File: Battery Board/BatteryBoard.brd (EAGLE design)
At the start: 40.6 x 80.5 mm, 38 parts, among them IC1 TPS63060DSCT, J0 1725656, J1 1725669, J2 UJ2-MIBH2-4-SMT-TR, J3 MPTC-02-16-02-6.30-XX-X-V, J4 JSTPH2, J5 MPTC-02-04-02-6.30-XX-X-V-LC, Q1 MMBTA56LT1G, Q2 MMBTA56LT1G, U0 STM32L031K4U6, U1 MCP73831T-2ATI_OT, U3 STM809TWX6F

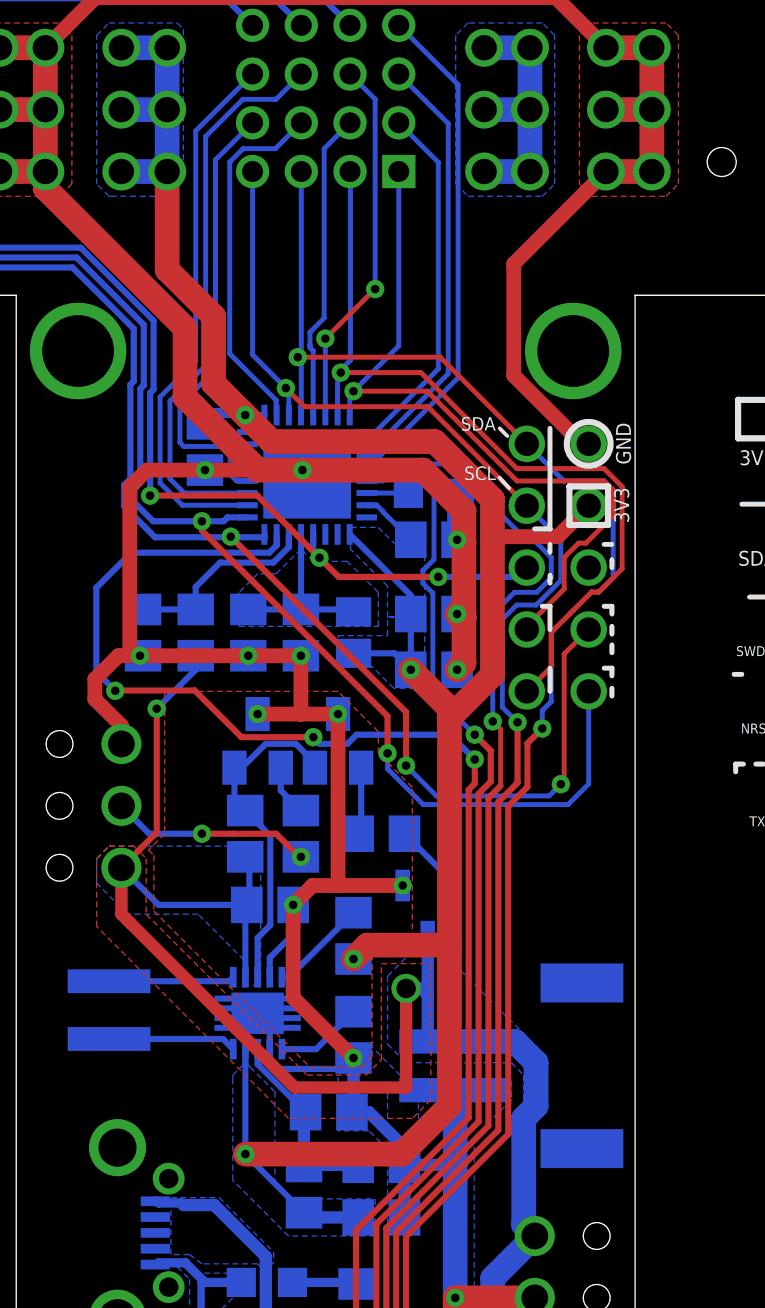
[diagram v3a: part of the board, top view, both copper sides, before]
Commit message: Started shield
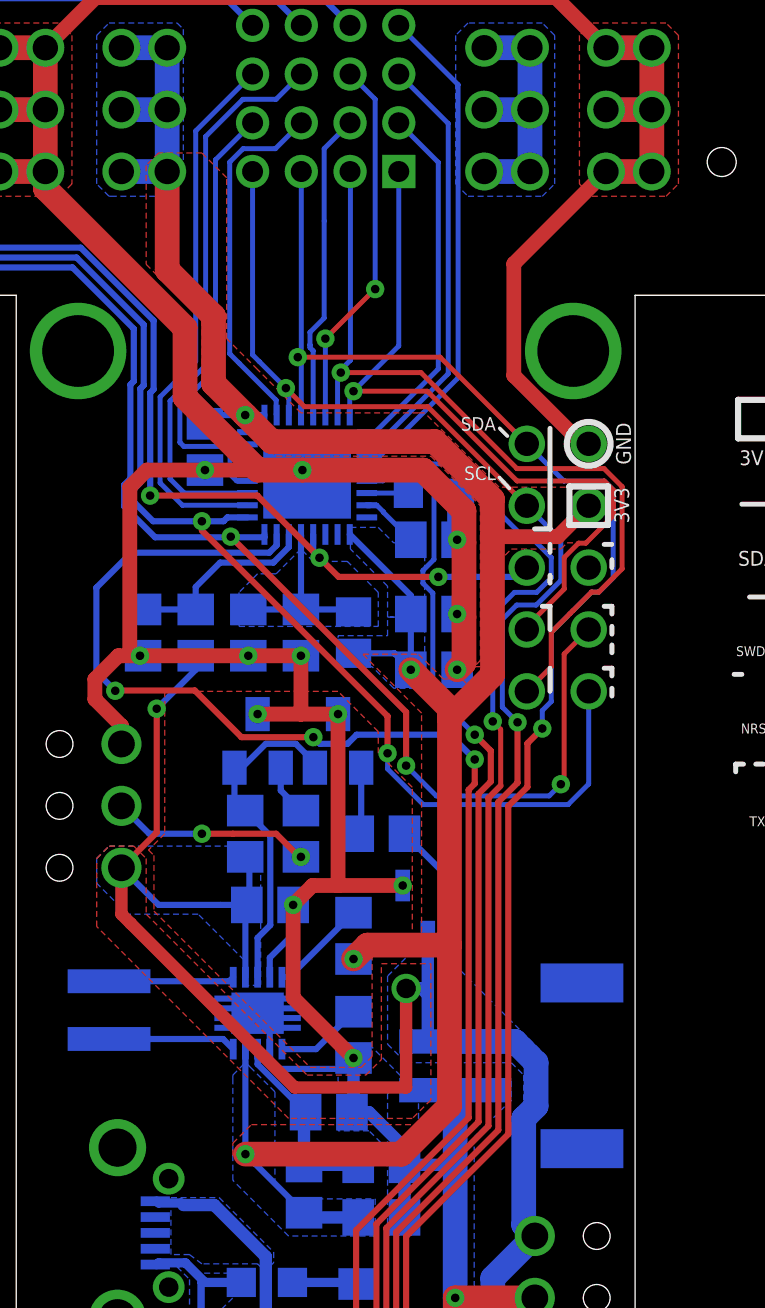
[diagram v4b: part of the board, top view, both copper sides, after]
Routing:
- net GND: track 273.5 -> 272.5 mm
- added copper zone on layer 1, net 3V3
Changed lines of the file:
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@@
 <setting verticaltext="up"/>
 </settings>
-<grid distance="10" unitdist="mil" unit="mil" style="lines" multiple="1" display="yes" altdistance="5" altunitdist="mil" altunit="mil"/>
+<grid distance="10" unitdist="mil" unit="mil" style="lines" multiple="1" display="yes" altdistance="125" altunitdist="mil" altunit="mil"/>
 <layers>
 <layer number="1" name="Top" color="4" fill="1" visible="yes" active="yes"/>
@@
 </polygon>
 <wire x1="-11.505" y1="30.226" x2="-11.505" y2="29.539" width="1.016" layer="1"/>
-<wire x1="11.43" y1="30.226" x2="11.505" y2="30.226" width="1.016" layer="1"/>
 <via x="10.795" y="19.05" extent="1-16" drill="1"/>
 <contactref element="Q1" pad="C"/>
@@
 <wire x1="-11.505" y1="29.539" x2="-5.7714" y2="23.8054" width="1.016" layer="1"/>
 <via x="-0.955" y="17.973" extent="1-16" drill="0.35"/>
-<wire x1="-0.955" y1="17.973" x2="-0.762" y2="17.78" width="1.016" layer="16"/>
-<wire x1="-0.762" y1="17.78" x2="-0.762" y2="17.018" width="1.016" layer="16"/>
 <via x="5.395" y="9.779" extent="1-16" drill="0.35"/>
 <wire x1="5.395" y1="9.779" x2="5.6762" y2="10.0602" width="1.016" layer="1"/>
 <wire x1="5.6762" y1="10.0602" x2="5.6762" y2="11.938" width="1.016" layer="1"/>
-<wire x1="5.5492" y1="12.065" x2="5.6762" y2="11.938" width="1.016" layer="1"/>
-<wire x1="5.6762" y1="11.938" x2="5.522" y2="11.938" width="1.016" layer="1"/>
-<wire x1="5.522" y1="11.938" x2="5.395" y2="12.065" width="1.016" layer="1"/>
-<via x="5.395" y="12.065" extent="1-16" drill="0.35"/>
 <wire x1="5.6762" y1="11.938" x2="5.6762" y2="14.986" width="1.016" layer="1"/>
 <wire x1="5.495" y1="15.213" x2="5.495" y2="17.018" width="1.016" layer="16"/>
@@
 <wire x1="5.395" y1="15.113" x2="5.495" y2="15.213" width="0.6096" layer="16"/>
 <wire x1="5.6762" y1="16.29343125" x2="5.6762" y2="14.986" width="1.016" layer="1"/>
-<wire x1="-0.955" y1="17.973" x2="1.016" y2="17.973" width="1.016" layer="1"/>
-<wire x1="1.016" y1="17.973" x2="3.99663125" y2="17.973" width="1.016" layer="1"/>
+<wire x1="-0.955" y1="17.973" x2="3.99663125" y2="17.973" width="1.016" layer="1"/>
 <wire x1="3.99663125" y1="17.973" x2="5.6762" y2="16.29343125" width="1.016" layer="1"/>
+<wire x1="5.6762" y1="11.938" x2="5.5492" y2="12.065" width="0.2032" layer="1"/>
+<wire x1="5.5492" y1="12.065" x2="5.395" y2="12.065" width="0.2032" layer="1"/>
+<via x="5.395" y="12.065" extent="1-16" drill="0.35"/>
+<wire x1="-0.762" y1="17.78" x2="-0.955" y2="17.973" width="0.2032" layer="16"/>
 </signal>
 <signal name="VDDA">
@@
 <wire x1="-17.993" y1="29.423" x2="-15.6718" y2="27.1018" width="0.254" layer="16"/>
 <via x="8.255" y="13.97" extent="1-16" drill="1"/>
-<wire x1="-0.508" y1="15.326" x2="-0.512" y2="15.33" width="0.254" layer="16"/>
-<wire x1="-0.512" y1="15.33" x2="-0.512" y2="14.863" width="0.1778" layer="16"/>
 <via x="-0.254" y="14.3744" extent="1-16" drill="0.35"/>
 <wire x1="-0.512" y1="15.33" x2="-0.512" y2="14.6324" width="0.254" layer="16"/>
@@
 <contactref element="J3" pad="P03_4"/>
 <wire x1="5.08" y1="-8.128" x2="5.08" y2="-1.524" width="1.016" layer="1"/>
-<wire x1="-6.35" y1="30.071" x2="-6.505" y2="30.226" width="1.016" layer="16"/>
 <wire x1="0.992" y1="15.33" x2="0.988" y2="15.33" width="0.254" layer="16"/>
 <polygon width="0.254" layer="16" thermals="no">
@@
 <wire x1="6.8446" y1="9.56080625" x2="5.08" y2="7.79620625" width="1.016" layer="1"/>
 <wire x1="6.8446" y1="9.56080625" x2="6.8446" y2="15.24" width="1.016" layer="1"/>
-<wire x1="-4.953" y1="19.873" x2="-4.953" y2="19.8984" width="1.016" layer="16"/>
 <via x="-3.302" y="20.23" extent="1-16" drill="0.35"/>
 <wire x1="-3.302" y1="20.23" x2="-4.603" y2="21.531" width="1.016" layer="1"/>
@@
 <wire x1="3.495" y1="9.779" x2="5.08" y2="8.194" width="1.016" layer="1"/>
 <wire x1="5.08" y1="8.194" x2="5.08" y2="7.79620625" width="1.016" layer="1"/>
+<polygon width="0.2032" layer="1">
+<vertex x="3.937" y="-1.397"/>
+<vertex x="3.937" y="8.001"/>
+<vertex x="1.524" y="10.414"/>
+<vertex x="3.81" y="10.414"/>
+<vertex x="4.826" y="9.398"/>
+<vertex x="5.588" y="9.398"/>
+<vertex x="6.096" y="9.906"/>
+<vertex x="7.112" y="9.906"/>
+<vertex x="5.08" y="7.874"/>
+<vertex x="5.08" y="-8.382"/>
+<vertex x="3.048" y="-10.414"/>
+<vertex x="-3.556" y="-10.414"/>
+<vertex x="-3.81" y="-10.16"/>
+<vertex x="-3.81" y="-9.652"/>
+<vertex x="-3.048" y="-8.89"/>
+<vertex x="3.81" y="-8.89"/>
+<vertex x="4.7625" y="-7.9375"/>
+<vertex x="4.7625" y="-2.2225"/>
+</polygon>
+<polygon width="0.2032" layer="1">
+<vertex x="7.366" y="14.478"/>
+<vertex x="7.62" y="14.732"/>
+<vertex x="9.652" y="14.732"/>
+<vertex x="9.906" y="14.986"/>
+<vertex x="10.668" y="14.986"/>
+<vertex x="11.684" y="16.002"/>
+<vertex x="11.684" y="16.764"/>
+<vertex x="11.684" y="17.018"/>
+<vertex x="11.43" y="17.272"/>
+<vertex x="7.874" y="17.272"/>
+<vertex x="7.112" y="17.272"/>
+<vertex x="6.858" y="17.526"/>
+<vertex x="4.064" y="20.32"/>
+<vertex x="3.81" y="20.32"/>
+<vertex x="-1.016" y="20.32"/>
+<vertex x="-2.794" y="22.098"/>
+<vertex x="-4.064" y="23.368"/>
+<vertex x="-4.064" y="29.972"/>
+<vertex x="-5.08" y="30.988"/>
+<vertex x="-6.858" y="30.988"/>
+<vertex x="-7.366" y="30.48"/>
+<vertex x="-7.366" y="29.718"/>
+<vertex x="-7.366" y="26.416"/>
+<vertex x="-6.858" y="25.908"/>
+<vertex x="-5.08" y="24.13"/>
+<vertex x="-5.08" y="21.844"/>
+<vertex x="-5.08" y="21.59"/>
+<vertex x="-2.286" y="18.796"/>
+<vertex x="-2.032" y="18.542"/>
+<vertex x="4.318" y="18.542"/>
+<vertex x="6.35" y="16.51"/>
+<vertex x="6.35" y="10.16"/>
+<vertex x="5.588" y="9.398"/>
+<vertex x="6.096" y="8.89"/>
+<vertex x="6.858" y="9.652"/>
+<vertex x="6.858" y="11.43"/>
+<vertex x="6.858" y="13.97"/>
+</polygon>
 </signal>
 <signal name="N$12">
@@
 <wire x1="-0.6442" y1="23.62986875" x2="-0.6442" y2="23.114" width="0.2032" layer="16"/>
 <wire x1="-0.6442" y1="23.114" x2="-0.6442" y2="23.10613125" width="0.2032" layer="16"/>
-<wire x1="-0.062" y1="31.164" x2="-0.062" y2="24.21206875" width="0.2032" layer="16"/>
+<wire x1="-0.062" y1="31.164" x2="-0.062" y2="28.194" width="0.2032" layer="16"/>
+<wire x1="-0.062" y1="28.194" x2="-0.062" y2="24.21206875" width="0.2032" layer="16"/>
 <wire x1="-0.062" y1="24.21206875" x2="-0.6442" y2="23.62986875" width="0.2032" layer="16"/>
 <wire x1="1" y1="32.226" x2="-0.062" y2="31.164" width="0.2032" layer="16"/>
